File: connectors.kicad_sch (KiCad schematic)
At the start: 35 parts, among them J10 Conn_01x06, J11 Conn_01x04, J12 USB4085-GF-A, J13 Conn_01x03, J14 Conn_01x03, J6 FTSH-107-01-L-DV-K-TR, J7 Conn_01x03, J8 Conn_01x02, J9 Conn_01x07, Q7 Si2302CDS

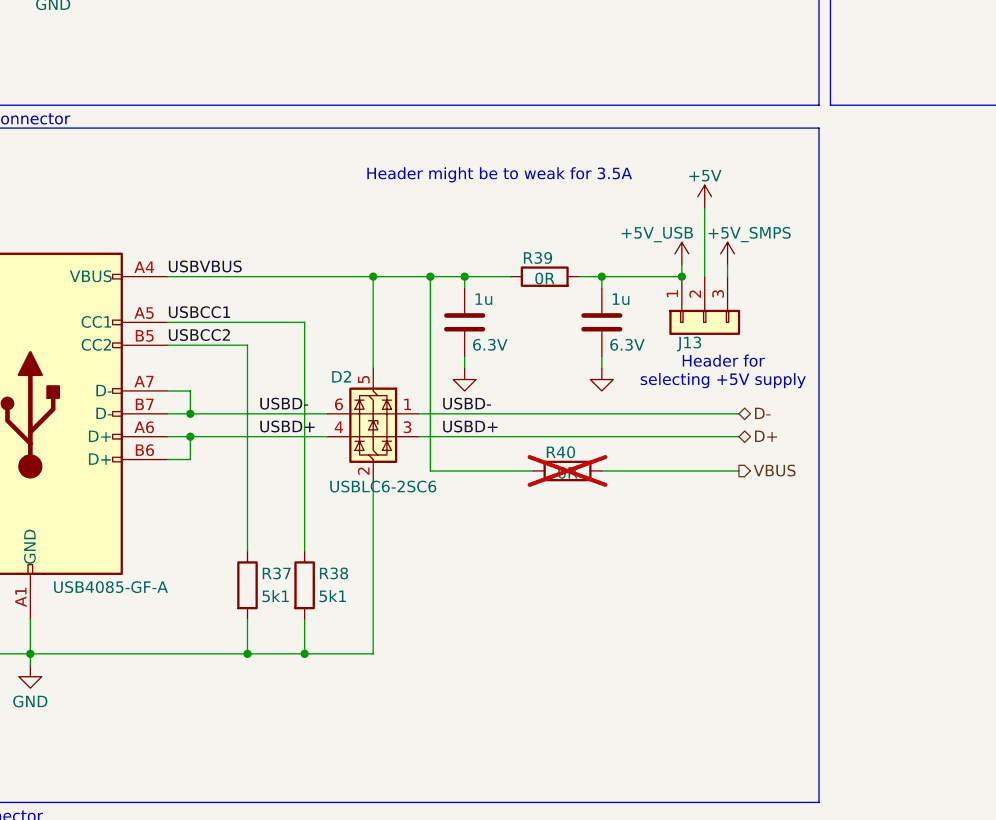
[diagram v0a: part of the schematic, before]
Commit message: WiP layout
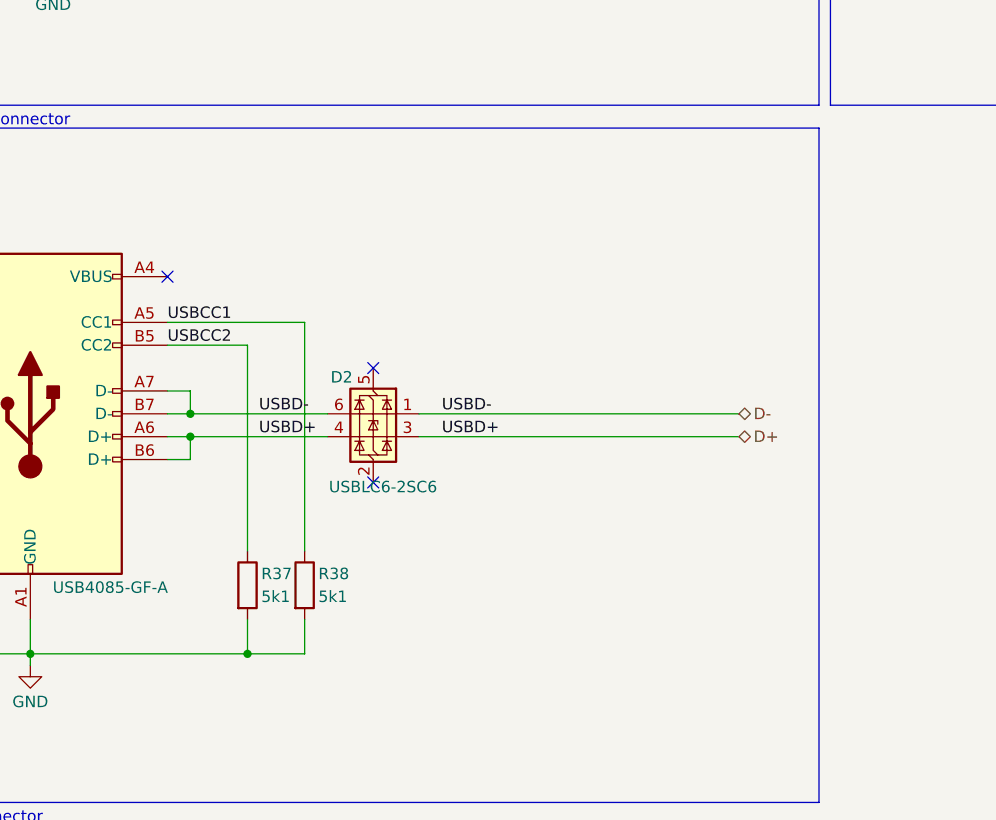
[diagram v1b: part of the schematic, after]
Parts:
- removed C67, C68: 1u, Capacitor_SMD:C_0402_1005Metric, symbol Device:C
- removed J13: Conn_01x03, Connector_PinHeader_1.00mm:PinHeader_1x03_P1.00mm_Vertical, symbol Connector_Generic:Conn_01x03
- removed R39, R40: 0R, Resistor_SMD:R_0603_1608Metric, symbol Device:R
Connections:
- net GND: no longer D2.2 (GND)
- net USBVBUS: no longer names the net of J12.A4 (VBUS), J12.A9 (VBUS), J12.B4 (VBUS), J12.B9 (VBUS)
- net USBVBUS: no longer D2.5 (VBUS)
- no-connect marks 4 -> 7
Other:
- note removed: "Header for selecting +5V supply"
- note removed: "Header might be to weak for 3.5A"
